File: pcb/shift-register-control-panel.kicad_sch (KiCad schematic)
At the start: 30 parts, among them J1 Conn_01x08, J2 USB_A, SW1 INPUT, SW2 SHIFT, SW3 CLEAR, SW4 DISPLAY, U1 74HC595, U2 LM7805_TO220

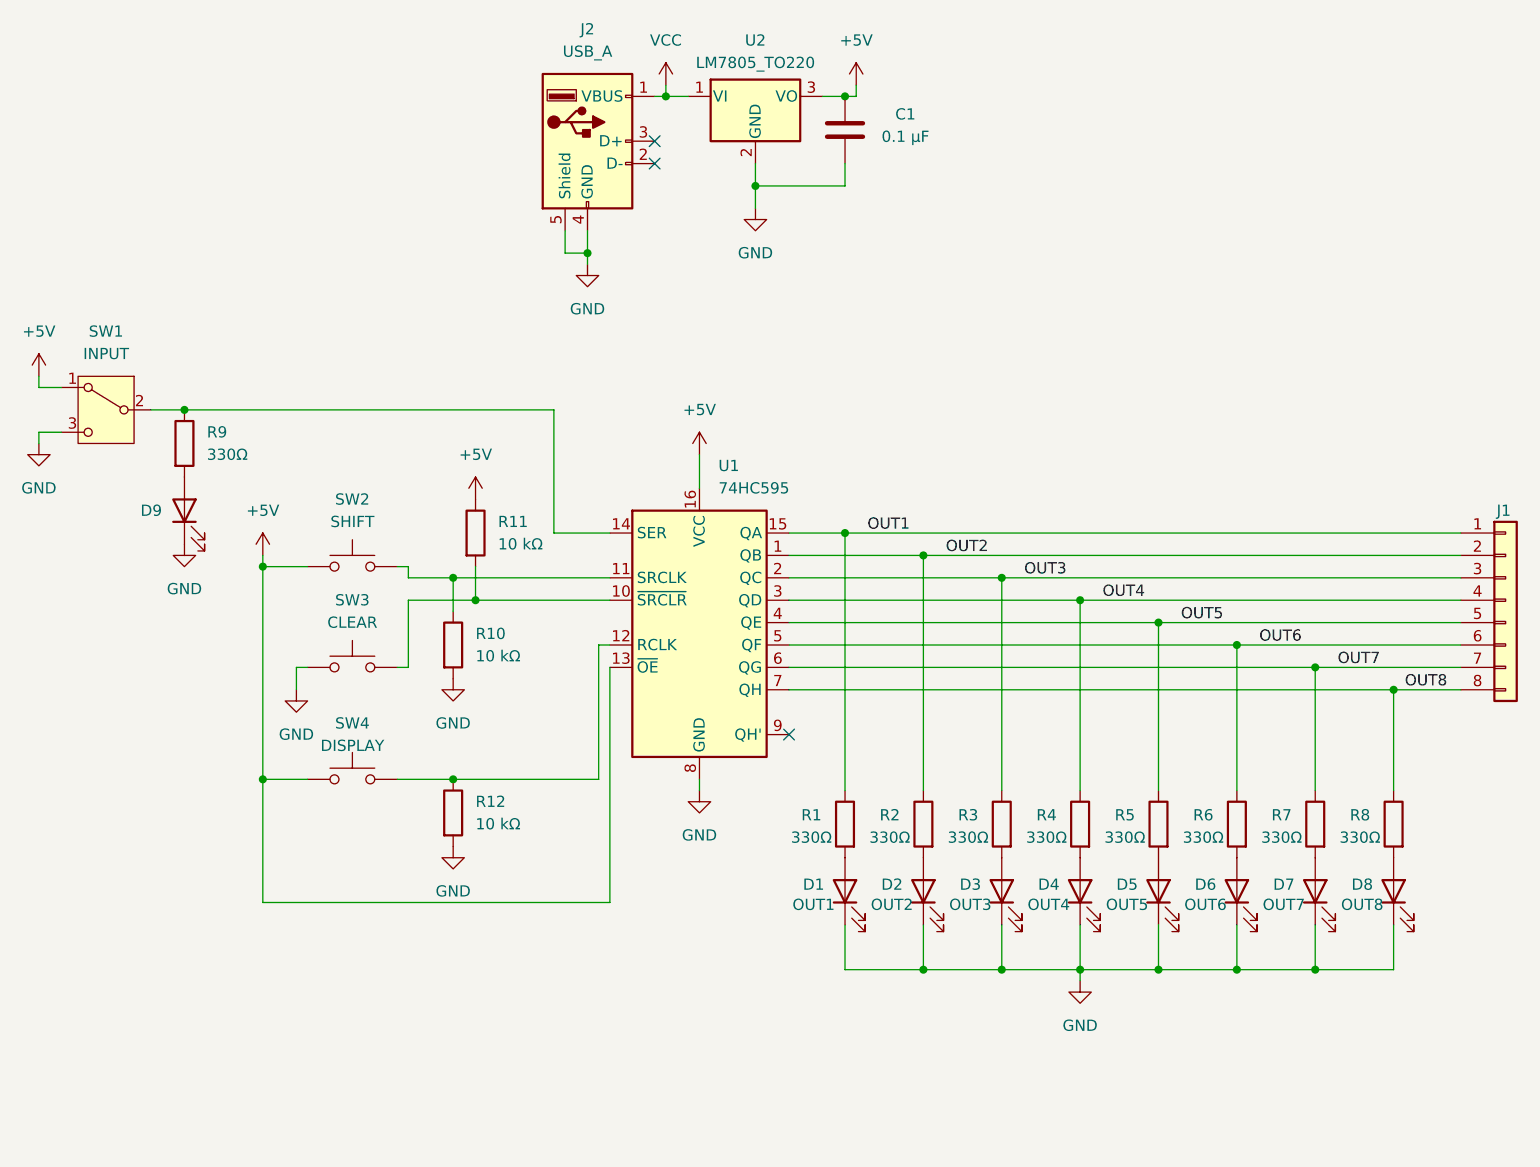
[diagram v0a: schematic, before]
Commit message: added assets
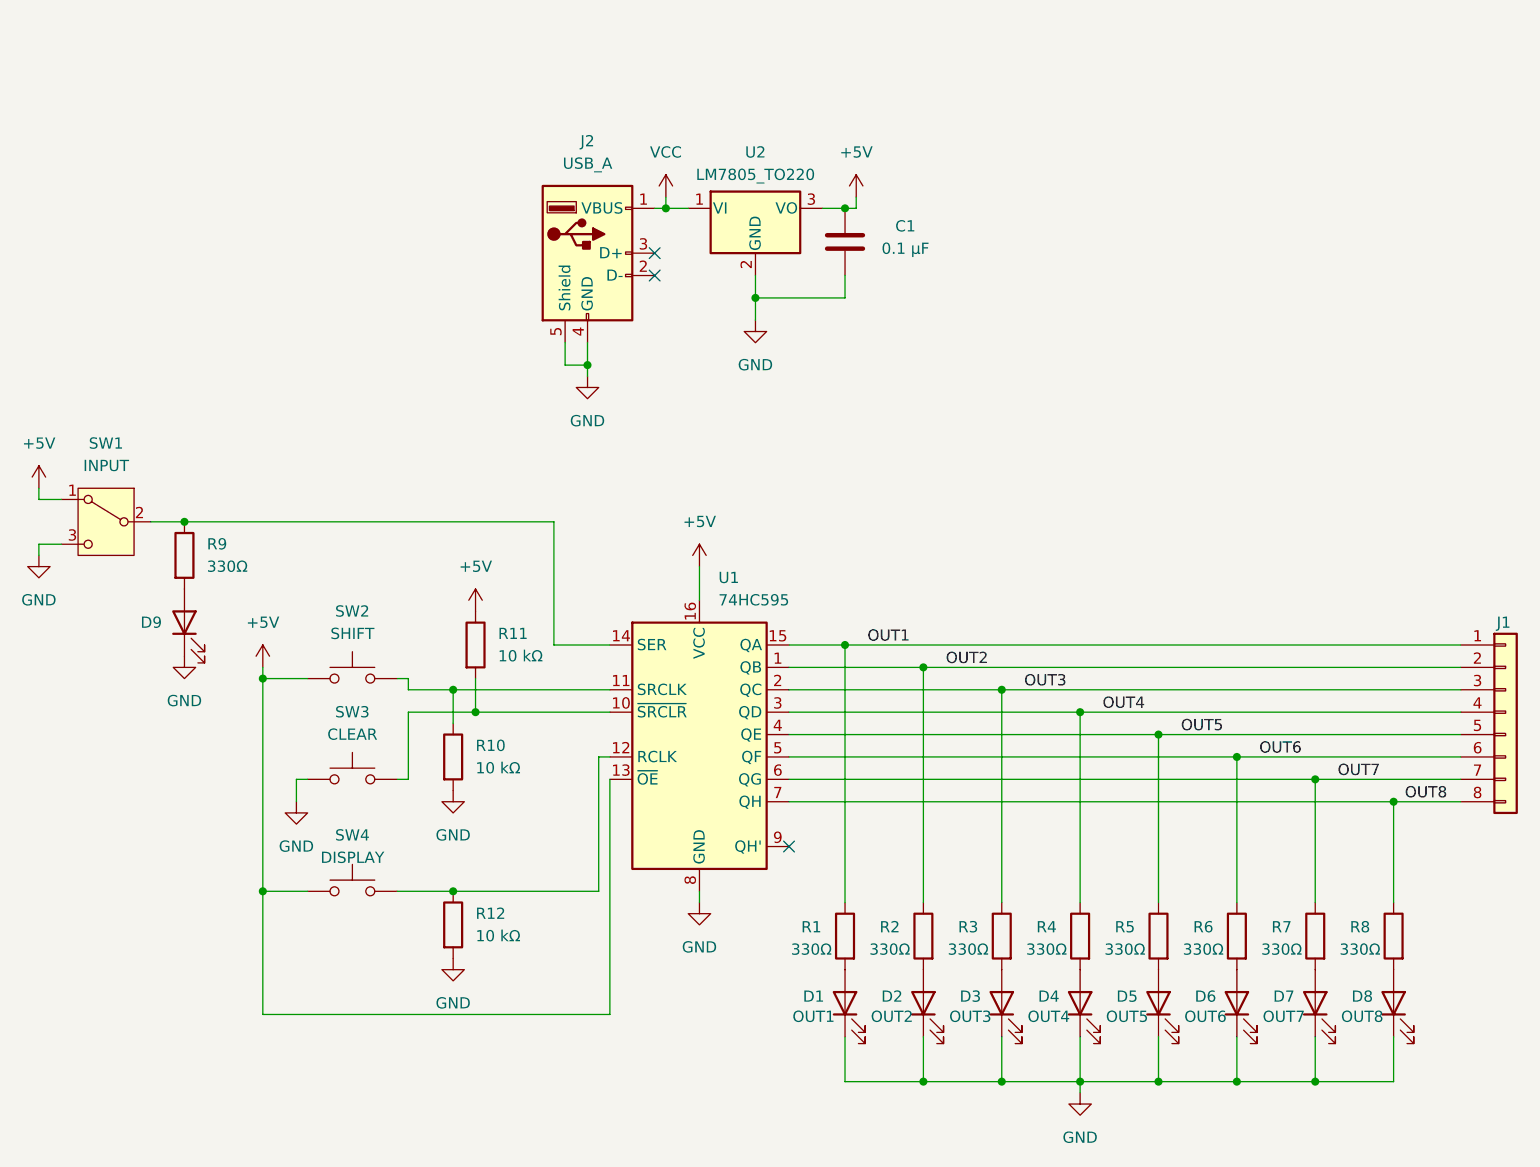
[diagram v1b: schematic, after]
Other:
- company: (none) -> The Metrobots
- title: (none) -> Shift Reigster Control Panel
- moved on the sheet: C1, D1, D2, D3, D4, D5, D6, D7, D8, D9, J1, J2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
